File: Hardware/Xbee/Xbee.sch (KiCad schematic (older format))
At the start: 36 parts, among them J1 Alimentación, J2 Raspberry, J3 Pines 1, J4 Pines 2, J5 Programación, J6 Entrada, J7 Salida, K1 SANYOU_SRD_Form_C, Q1 2N7002, Q2 AP2300, SW1 Reset, SW2 Comm., U2 Xbee, U3 LM358

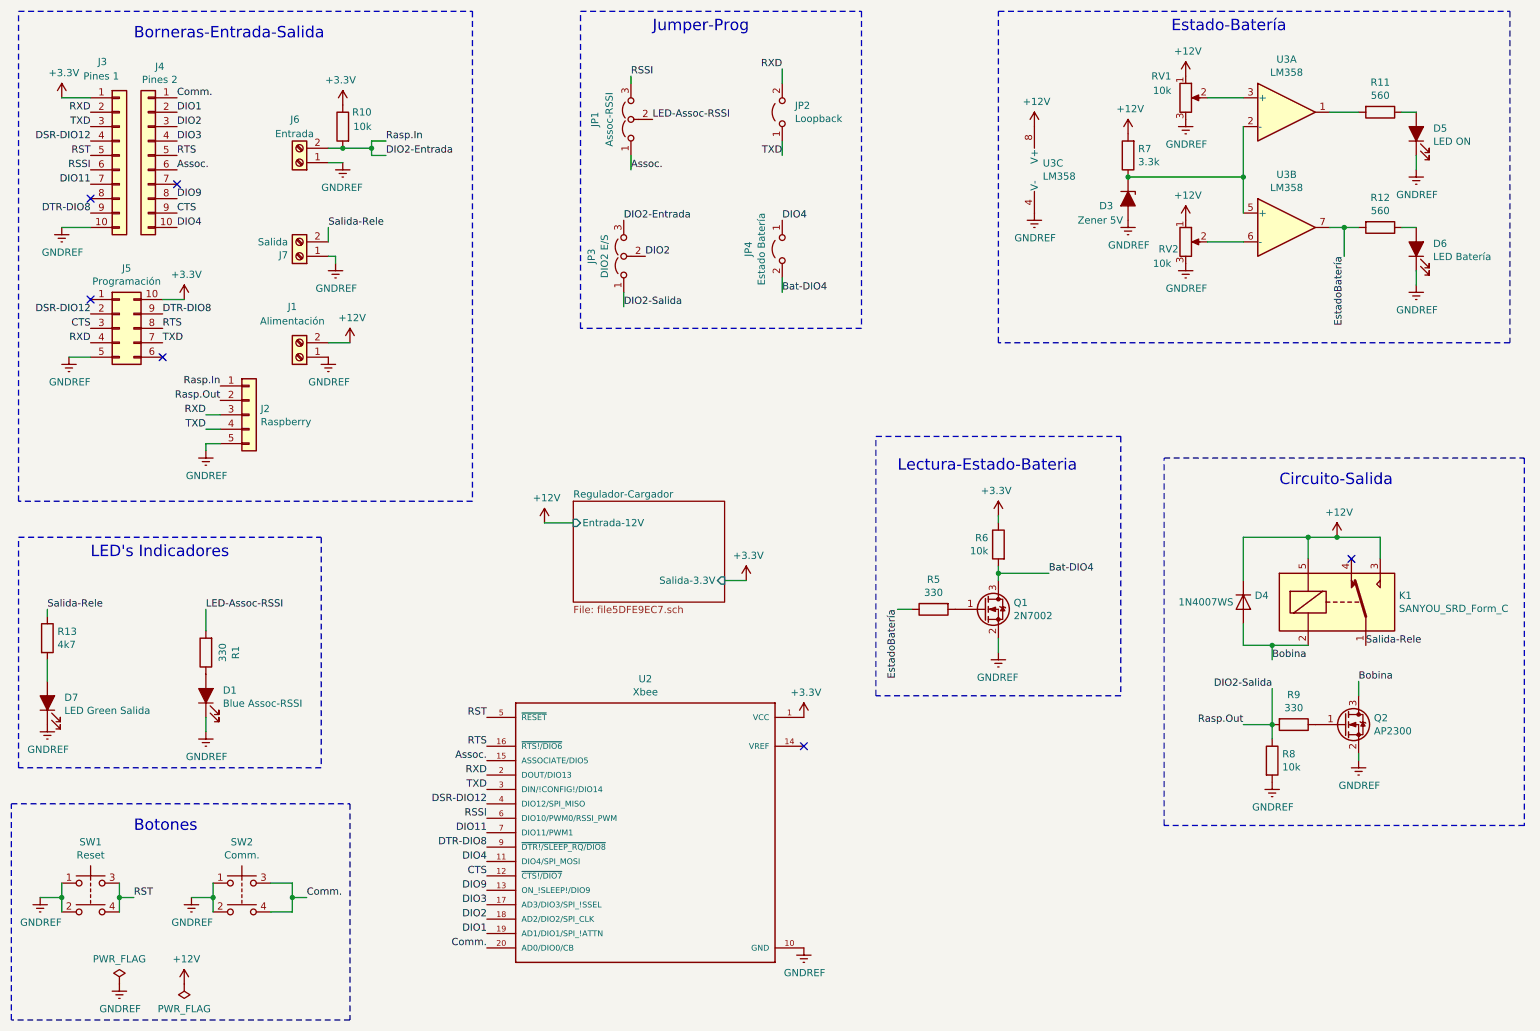
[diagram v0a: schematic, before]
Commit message: Battery Charger
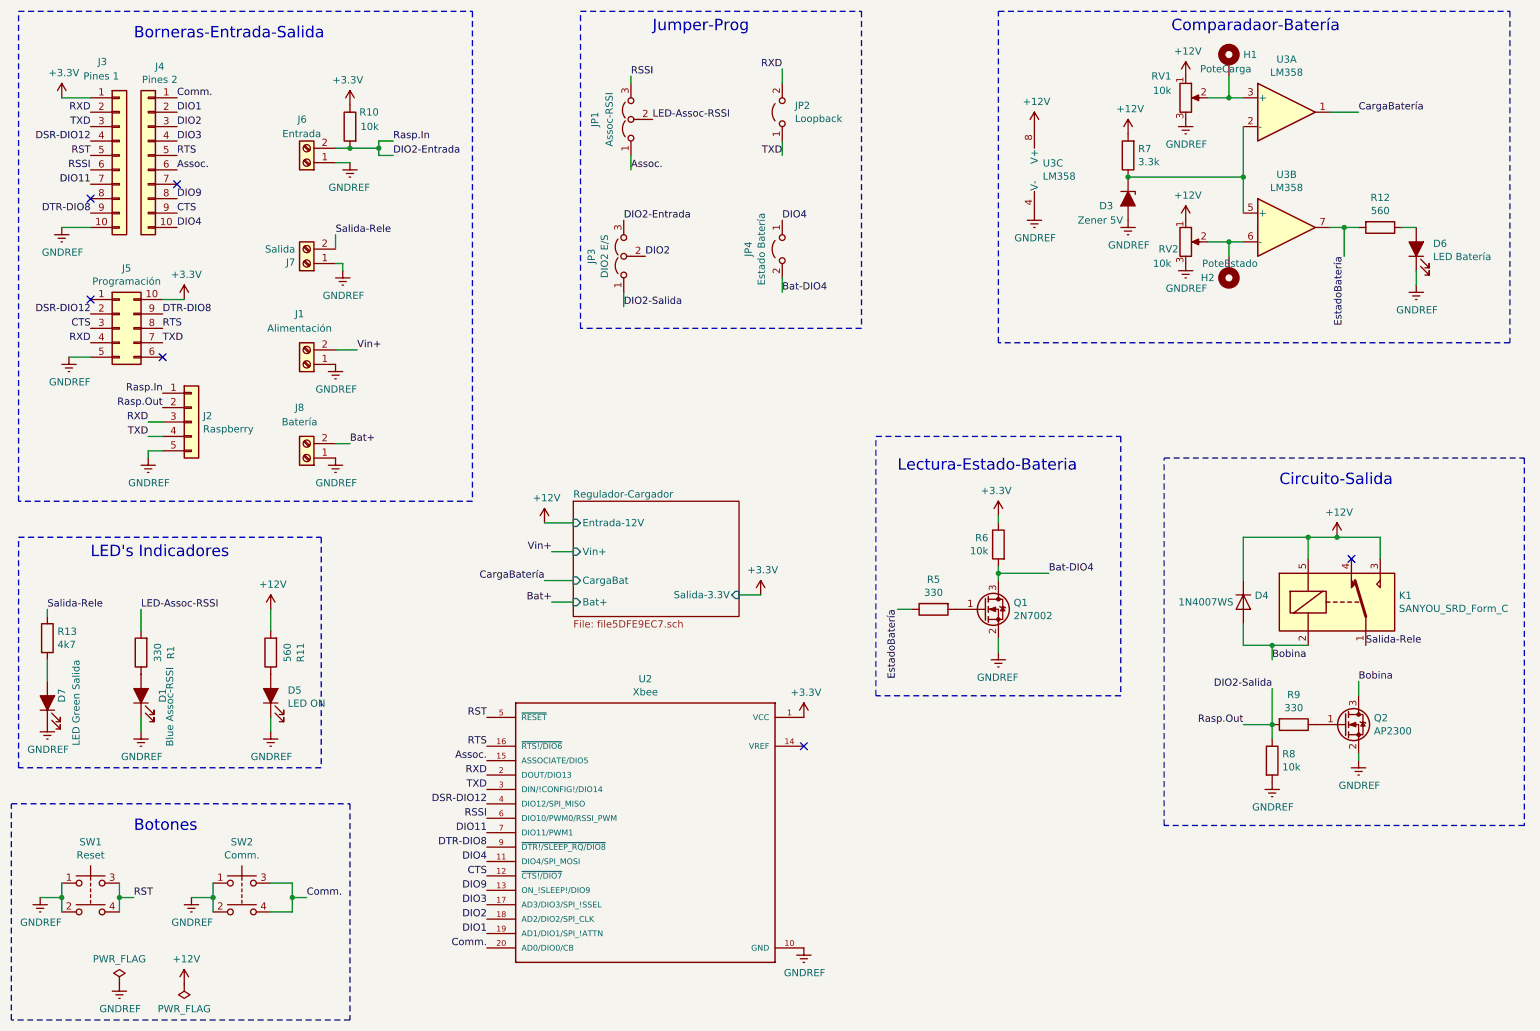
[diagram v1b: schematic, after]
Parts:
- added H1: PoteCarga, symbol Mechanical:MountingHole_Pad
- added H2: PoteEstado, symbol Mechanical:MountingHole_Pad
- added J8: Batería, TerminalBlock:TerminalBlock_bornier-2_P5.08mm, symbol Xbee-rescue:Screw_Terminal_01x02-Connector
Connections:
- net +12V: now also R11.2; no longer J1.2 (Pin_2)
- net GNDREF: now also J8.1 (Pin_1)
- net at RV1.2, U3.3 (+): now also H1.1
- net at RV2.2, U3.6 (-): now also H2.1
- net CargaBatería: now reaches U3.1
- net CargaBatería: no longer R11.2
- new net Bat+: J8.2 (Pin_2)
- new net Vin+: J1.2 (Pin_2)
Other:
- note added: "Comparadaor-Batería"
- note removed: "Estado-Batería"
- moved on the sheet: D1, D5, J1, J2, J6, J7, R1, R10, R11
